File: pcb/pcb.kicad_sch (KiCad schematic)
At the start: 16 parts, among them CN10 1x2, CN2 1x8, CN3 1x8, CN4 1x8, CN5 1x4, CN6 1x2, CN7 1x2, SW1 switch_3x4, SW2 switch_3x4

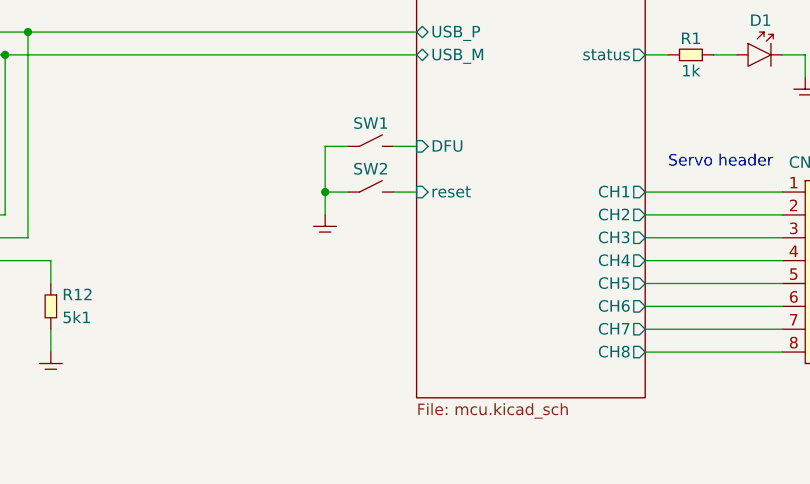
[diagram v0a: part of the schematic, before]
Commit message: added DIP switches, footprints
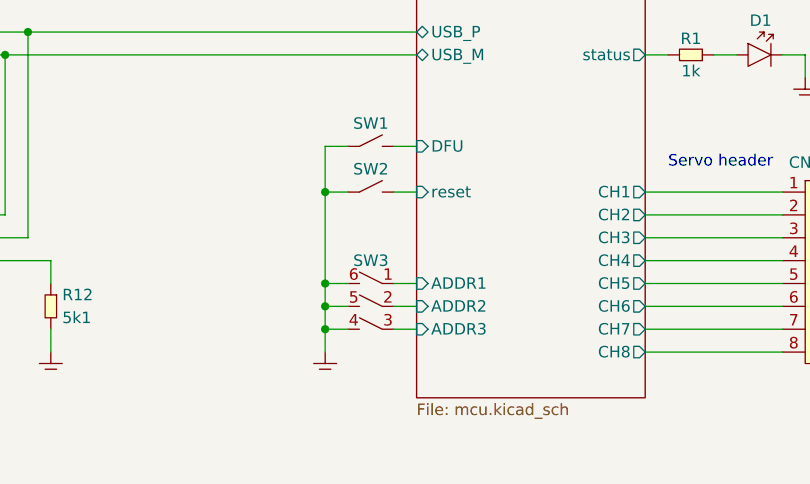
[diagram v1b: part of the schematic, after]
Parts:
- added SW3: 219-3LPST, buttons:219-3LPST, symbol switches:219-3LPST
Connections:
- net GND: now also SW3.4, SW3.5, SW3.6
- new net MCU/ADDR1: SW3.1
- new net MCU/ADDR2: SW3.2
- new net MCU/ADDR3: SW3.3
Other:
- sheet MCU ports: added ADDR1, ADDR2, ADDR3; removed none
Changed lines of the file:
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@@
   (junction (at 190.5 137.16) (diameter 0) (color 0 0 0 0)
   )
+  (junction (at 129.54 134.62) (diameter 0) (color 0 0 0 0)
+  )
   (junction (at 76.2 147.32) (diameter 0) (color 0 0 0 0)
   )
@@
   (junction (at 203.2 132.08) (diameter 0) (color 0 0 0 0)
   )
+  (junction (at 129.54 137.16) (diameter 0) (color 0 0 0 0)
+  )
   (junction (at 73.66 147.32) (diameter 0) (color 0 0 0 0)
   )
@@
   (junction (at 93.98 106.68) (diameter 0) (color 0 0 0 0)
   )
+  (junction (at 129.54 132.08) (diameter 0) (color 0 0 0 0)
+  )
   (junction (at 78.74 147.32) (diameter 0) (color 0 0 0 0)
   )
@@
     (stroke (width 0) (type default))
   )
+  (wire (pts (xy 129.54 134.62) (xy 132.08 134.62))
+    (stroke (width 0) (type default))
+  )
   (wire (pts (xy 203.2 121.92) (xy 205.74 121.92))
     (stroke (width 0) (type default))
@@
     (stroke (width 0) (type default))
   )
+  (wire (pts (xy 129.54 132.08) (xy 129.54 121.92))
+    (stroke (width 0) (type default))
+  )
   (wire (pts (xy 203.2 137.16) (xy 205.74 137.16))
     (stroke (width 0) (type default))
@@
     (stroke (width 0) (type default))
   )
+  (wire (pts (xy 129.54 134.62) (xy 129.54 132.08))
+    (stroke (width 0) (type default))
+  )
   (wire (pts (xy 165.1 106.68) (xy 167.64 106.68))
     (stroke (width 0) (type default))
@@
     (stroke (width 0) (type default))
   )
+  (wire (pts (xy 137.16 132.08) (xy 139.7 132.08))
+    (stroke (width 0) (type default))
+  )
   (wire (pts (xy 203.2 124.46) (xy 205.74 124.46))
     (stroke (width 0) (type default))
@@
     (stroke (width 0) (type default))
   )
+  (wire (pts (xy 129.54 132.08) (xy 132.08 132.08))
+    (stroke (width 0) (type default))
+  )
   (wire (pts (xy 190.5 127) (xy 193.04 127))
     (stroke (width 0) (type default))
@@
     (stroke (width 0) (type default))
   )
+  (wire (pts (xy 137.16 137.16) (xy 139.7 137.16))
+    (stroke (width 0) (type default))
+  )
   (wire (pts (xy 190.5 124.46) (xy 190.5 127))
     (stroke (width 0) (type default))
@@
     (stroke (width 0) (type default))
   )
+  (wire (pts (xy 129.54 137.16) (xy 129.54 134.62))
+    (stroke (width 0) (type default))
+  )
+  (wire (pts (xy 129.54 137.16) (xy 132.08 137.16))
+    (stroke (width 0) (type default))
+  )
   (wire (pts (xy 129.54 121.92) (xy 132.08 121.92))
     (stroke (width 0) (type default))
@@
     (stroke (width 0) (type default))
   )
-  (wire (pts (xy 129.54 124.46) (xy 129.54 121.92))
+  (wire (pts (xy 129.54 139.7) (xy 129.54 137.16))
     (stroke (width 0) (type default))
   )
@@
   )
   (wire (pts (xy 78.74 147.32) (xy 78.74 149.86))
+    (stroke (width 0) (type default))
+  )
+  (wire (pts (xy 137.16 134.62) (xy 139.7 134.62))
     (stroke (width 0) (type default))
   )
@@
     )
   )
-  (symbol (lib_id "generic:GND") (at 129.54 124.46 0) (unit 1)
-    (in_bom yes) (on_board yes) (dnp no) (fields_autoplaced)
-    (property "Reference" "#GND01" (at 133.35 123.19 0)
-      (effects (font (size 1.27 1.27)) hide)
-    )
-    (property "Value" "GND" (at 133.35 124.46 0)
-      (effects (font (size 1.27 1.27)) hide)
-    )
-    (property "Footprint" "" (at 129.54 124.46 0)
-      (effects (font (size 1.27 1.27)) hide)
-    )
-    (property "Datasheet" "" (at 129.54 124.46 0)
+  (symbol (lib_id "generic:GND") (at 129.54 139.7 0) (unit 1)
+    (in_bom yes) (on_board yes) (dnp no) (fields_autoplaced)
+    (property "Reference" "#GND01" (at 133.35 138.43 0)
+      (effects (font (size 1.27 1.27)) hide)
+    )
+    (property "Value" "GND" (at 133.35 139.7 0)
+      (effects (font (size 1.27 1.27)) hide)
+    )
+    (property "Footprint" "" (at 129.54 139.7 0)
+      (effects (font (size 1.27 1.27)) hide)
+    )
+    (property "Datasheet" "" (at 129.54 139.7 0)
       (effects (font (size 1.27 1.27)) hide)
     )
@@
     )
   )
+  (symbol (lib_id "switches:219-3LPST") (at 134.62 132.08 0) (mirror y) (unit 1)
+    (in_bom yes) (on_board yes) (dnp no) (fields_autoplaced)
+    (property "Reference" "SW3" (at 134.62 129.54 0)
+      (effects (font (size 1.27 1.27)))
+    )
+    (property "Value" "219-3LPST" (at 134.62 125.73 0)
+      (effects (font (size 1.27 1.27)) hide)
+    )
+    (property "Footprint" "buttons:219-3LPST" (at 134.62 139.7 0)
+      (effects (font (size 1.27 1.27)) hide)
+    )
+    (property "Datasheet" "https://www.ctscorp.com/Files/DataSheets/Switches/DIP-Switches/CTS-Switches-DIP-219-Series-Datasheet.pdf" (at 135.89 124.46 0)
+      (effects (font (size 1.27 1.27)) hide)
+    )
+    (property "Digi-Key" "CT2193LPST-ND" (at 134.62 125.73 0)
+      (effects (font (size 1.27 1.27)) hide)
+    )
+    (property "MPN" "219-3LPST" (at 134.62 139.7 0)
+      (effects (font (size 1.27 1.27)) hide)
+    )
+    (pin "1")
+    (pin "2")
+    (pin "3")
+    (pin "4")
+    (pin "5")
+    (pin "6")
+    (instances
+      (project "pcb"
+        (path "/6bb3bad6-1a89-4624-b34d-6ddda7dd16d2"
+          (reference "SW3") (unit 1)
+        )
+      )
+    )
+  )
   (symbol (lib_name "GND_1") (lib_id "generic:GND") (at 58.42 139.7 0) (unit 1)
     (in_bom yes) (on_board yes) (dnp no) (fields_autoplaced)
@@
       (effects (font (size 1.27 1.27)) (justify left))
     )
+    (pin "ADDR3" input (at 139.7 137.16 180)
+      (effects (font (size 1.27 1.27)) (justify left))
+    )
+    (pin "ADDR2" input (at 139.7 134.62 180)
+      (effects (font (size 1.27 1.27)) (justify left))
+    )
+    (pin "ADDR1" input (at 139.7 132.08 180)
+      (effects (font (size 1.27 1.27)) (justify left))
+    )
